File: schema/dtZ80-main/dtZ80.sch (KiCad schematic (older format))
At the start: 9 parts, among them J1 PRPC040SAAN-RC, U1 Z80CPU, U2 28C256, U3 74LS32, X1 CXO_DIP8

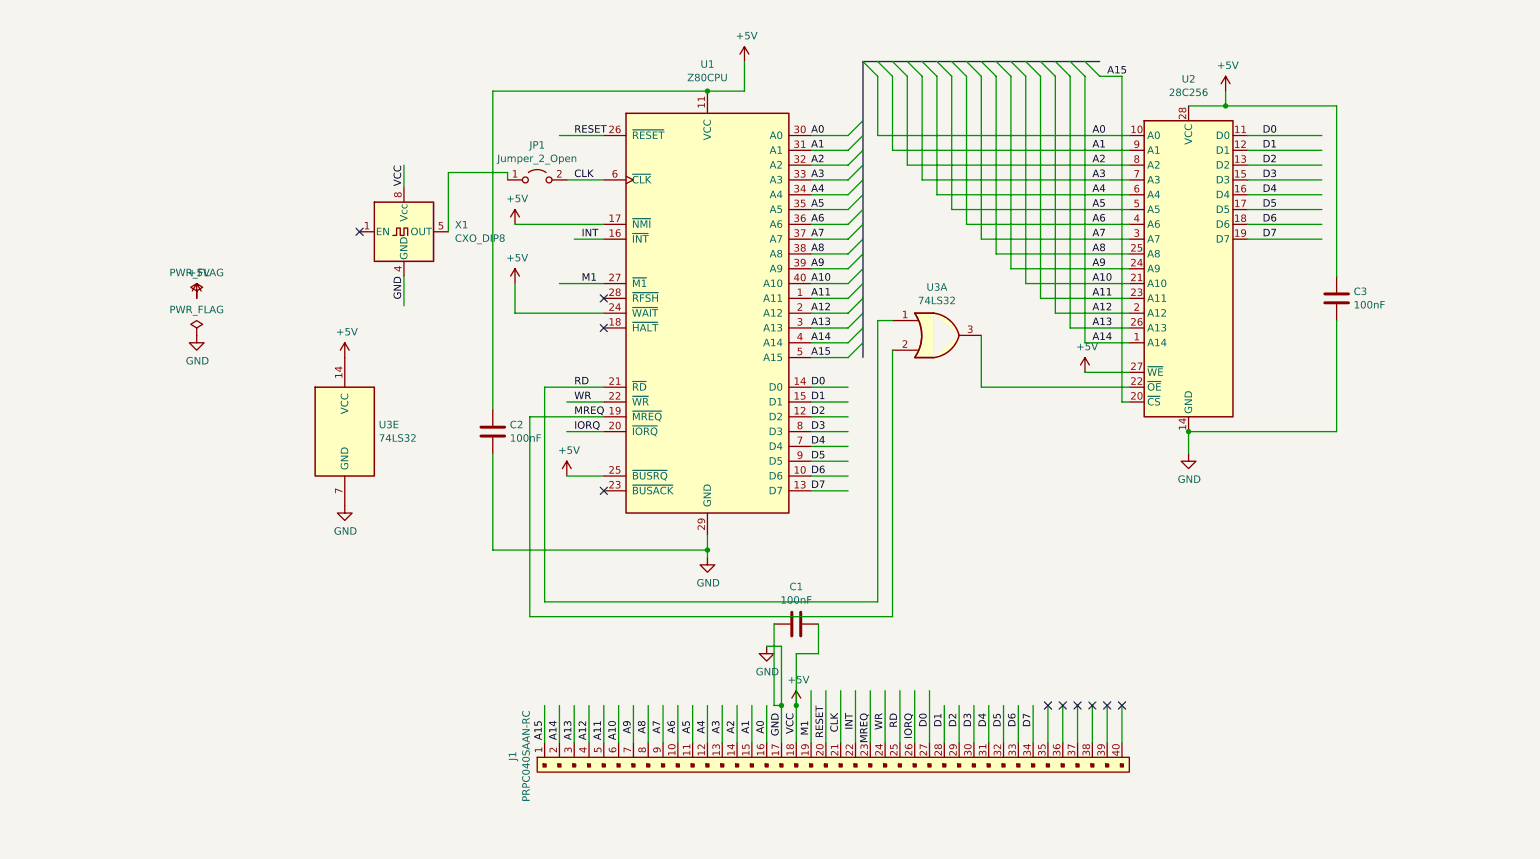
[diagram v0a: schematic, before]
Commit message: Reworked Boards
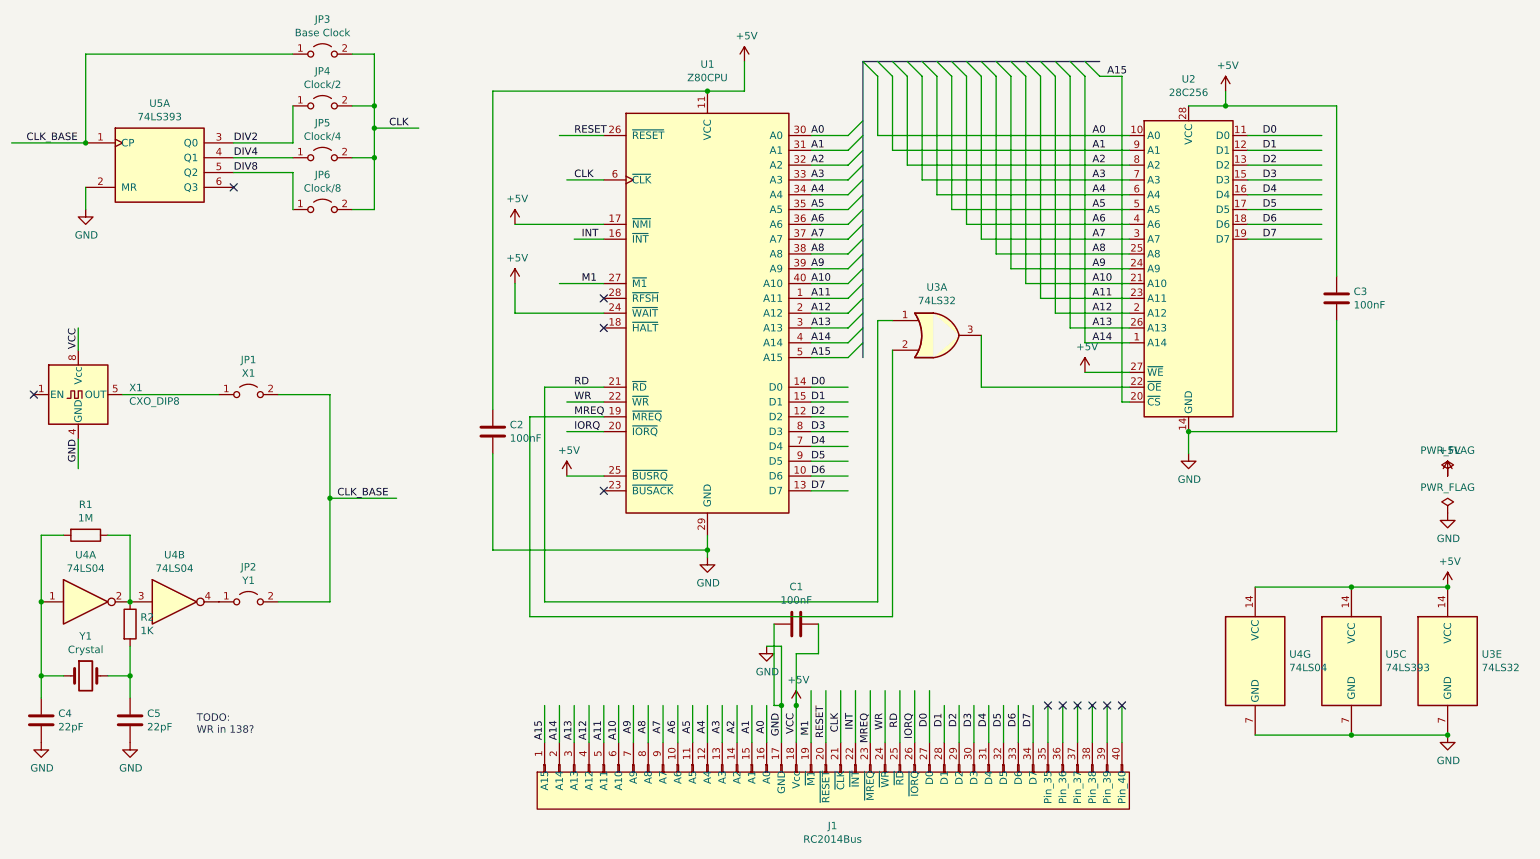
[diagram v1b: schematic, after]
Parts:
- removed J1: PRPC040SAAN-RC, Connector_PinHeader_2.54mm:PinHeader_1x40_P2.54mm_Vertical, symbol dk_Rectangular-Connectors-Headers-Male-Pins:PRPC040SAAN-RC
- added C4, C5: 22pF, Capacitor_THT:C_Disc_D4.3mm_W1.9mm_P5.00mm, symbol Device:C
- added J1: RC2014Bus, Connector_PinHeader_2.54mm:PinHeader_1x40_P2.54mm_Vertical, symbol rc2014bus:RC2014Bus
- added JP2: Y1, Connector_PinHeader_2.54mm:PinHeader_1x02_P2.54mm_Vertical, symbol Jumper:Jumper_2_Open
- added JP3: Base Clock, Connector_PinHeader_2.54mm:PinHeader_1x02_P2.54mm_Vertical, symbol Jumper:Jumper_2_Open
- added JP4: Clock/2, Connector_PinHeader_2.54mm:PinHeader_1x02_P2.54mm_Vertical, symbol Jumper:Jumper_2_Open
- added JP5: Clock/4, Connector_PinHeader_2.54mm:PinHeader_1x02_P2.54mm_Vertical, symbol Jumper:Jumper_2_Open
- added JP6: Clock/8, Connector_PinHeader_2.54mm:PinHeader_1x02_P2.54mm_Vertical, symbol Jumper:Jumper_2_Open
- added R1: 1M, Resistor_THT:R_Axial_DIN0204_L3.6mm_D1.6mm_P5.08mm_Horizontal, symbol Device:R
- added R2: 1K, Resistor_THT:R_Axial_DIN0204_L3.6mm_D1.6mm_P5.08mm_Horizontal, symbol Device:R
- added U4: 74LS04, Package_DIP:DIP-14_W7.62mm_Socket, symbol 74xx:74AHC04
- added U5: 74LS393, Package_DIP:DIP-14_W7.62mm_Socket, symbol 74xx:74LS393
- added Y1: Crystal, Crystal:Crystal_HC52-8mm_Vertical, symbol Device:Crystal
- JP1: value Jumper_2_Open -> X1
- U2: footprint Package_DIP:DIP-28_W15.24mm -> dtZ80-main:DIP-28_W15.24mm_Socket_Large_Holes
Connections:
- net labels added: CLK_BASE, DIV2, DIV4, DIV8
- wire segments 154 -> 189
- no-connect marks 10 -> 11
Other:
- note added: "TODO:\nWR in 138?"
- moved on the sheet: JP1, U3E, X1
